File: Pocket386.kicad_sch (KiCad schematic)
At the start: 19 parts, among them J1 Conn_02x40_Odd_Even, U1 Pico, U2 SN74CB3T3257, U3 SN74CB3T3257, U4 74AHC14, U5 74LVC00, U6 SN74CB3T3245, U7 APS6404L-3SQN-SN, U8 74LVC1G00, U9 74LVC1G06

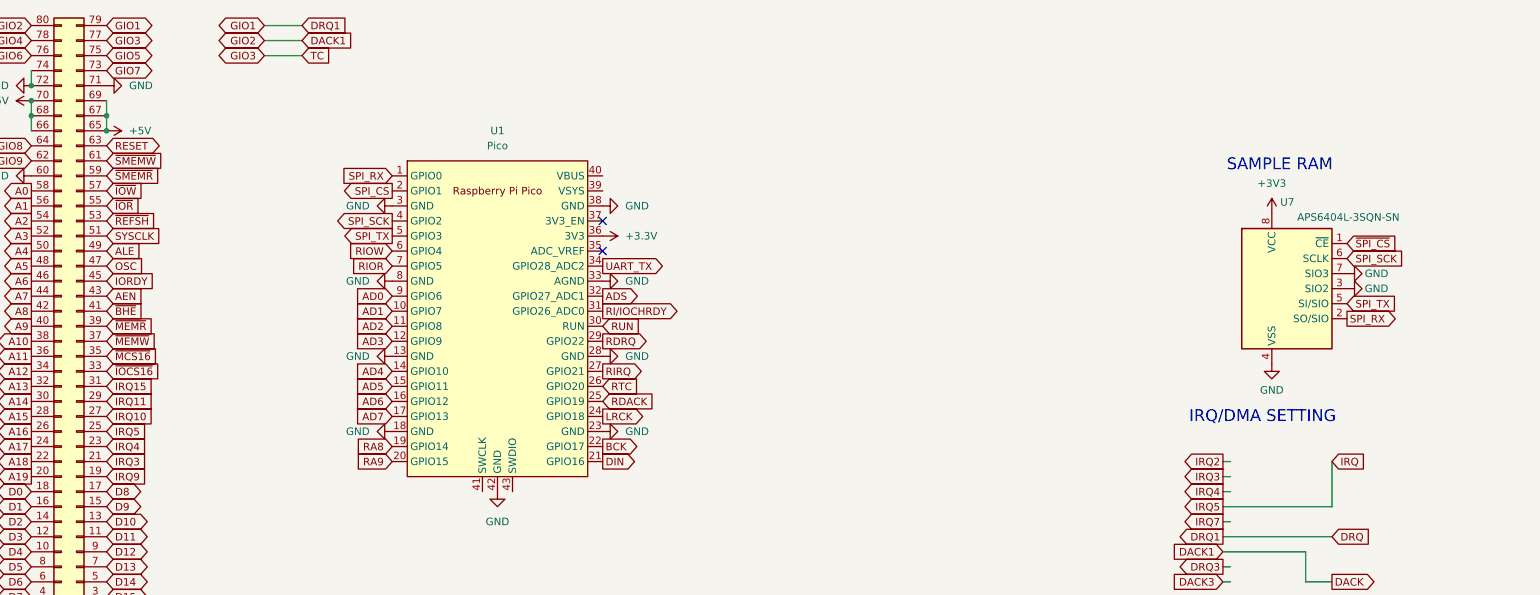
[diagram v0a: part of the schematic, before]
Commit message: Add back [final?] signals?
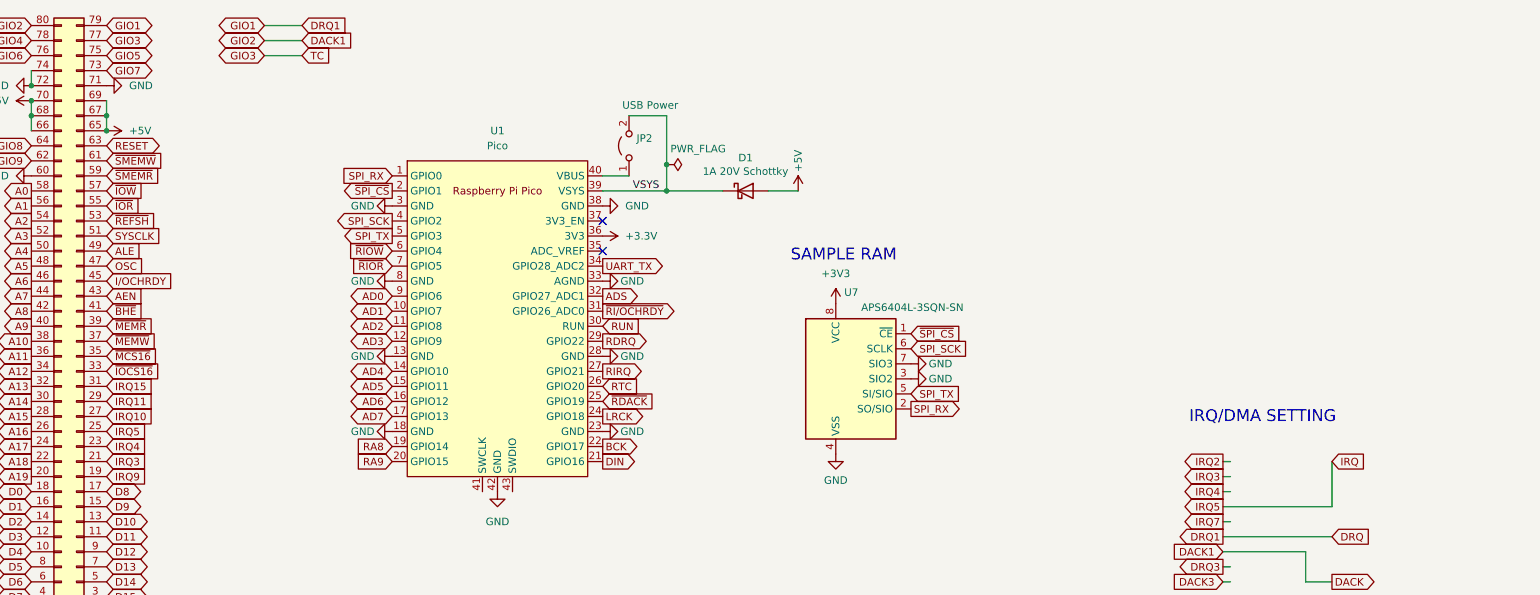
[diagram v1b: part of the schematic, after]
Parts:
- added D1: 1A 20V Schottky, Diode_SMD:D_SOD-123, symbol Device:D_Schottky
- added JP2: USB Power, Connector_PinHeader_2.54mm:PinHeader_1x02_P2.54mm_Vertical, symbol Jumper:Jumper_2_Open
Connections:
- net IORDY is gone; now on net I/OCHRDY: J1.45 (Pin_45)
- net RDACK is gone; now on net ~{RDACK}: U1.25 (GPIO19)
- net RIOR is gone; now on net ~{RIOR}: U1.7 (GPIO5)
- net RIOW is gone; now on net ~{RIOW}: U1.6 (GPIO4)
- net RI/IOCHRDY is gone; now on net ~{RI/OCHRDY}: U1.31 (GPIO26_ADC0)
- net SPI_CS is gone; now on net ~{SPI_CS}: U1.2 (GPIO1)
- net +5V: now also D1.2 (A)
- net VSYS: now reaches U1.39 (VSYS)
- net VSYS: now also D1.1 (K), JP2.2 (B)
- net at U1.40 (VBUS): now also JP2.1 (A)
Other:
- moved on the sheet: U7
